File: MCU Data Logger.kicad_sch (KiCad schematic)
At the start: 25 parts, among them U1 24LC1025, U2 24LC1025, U3 DS1337S_, U4 ATmega328P-A, Y1 32.768KHz, Y2 16MHz

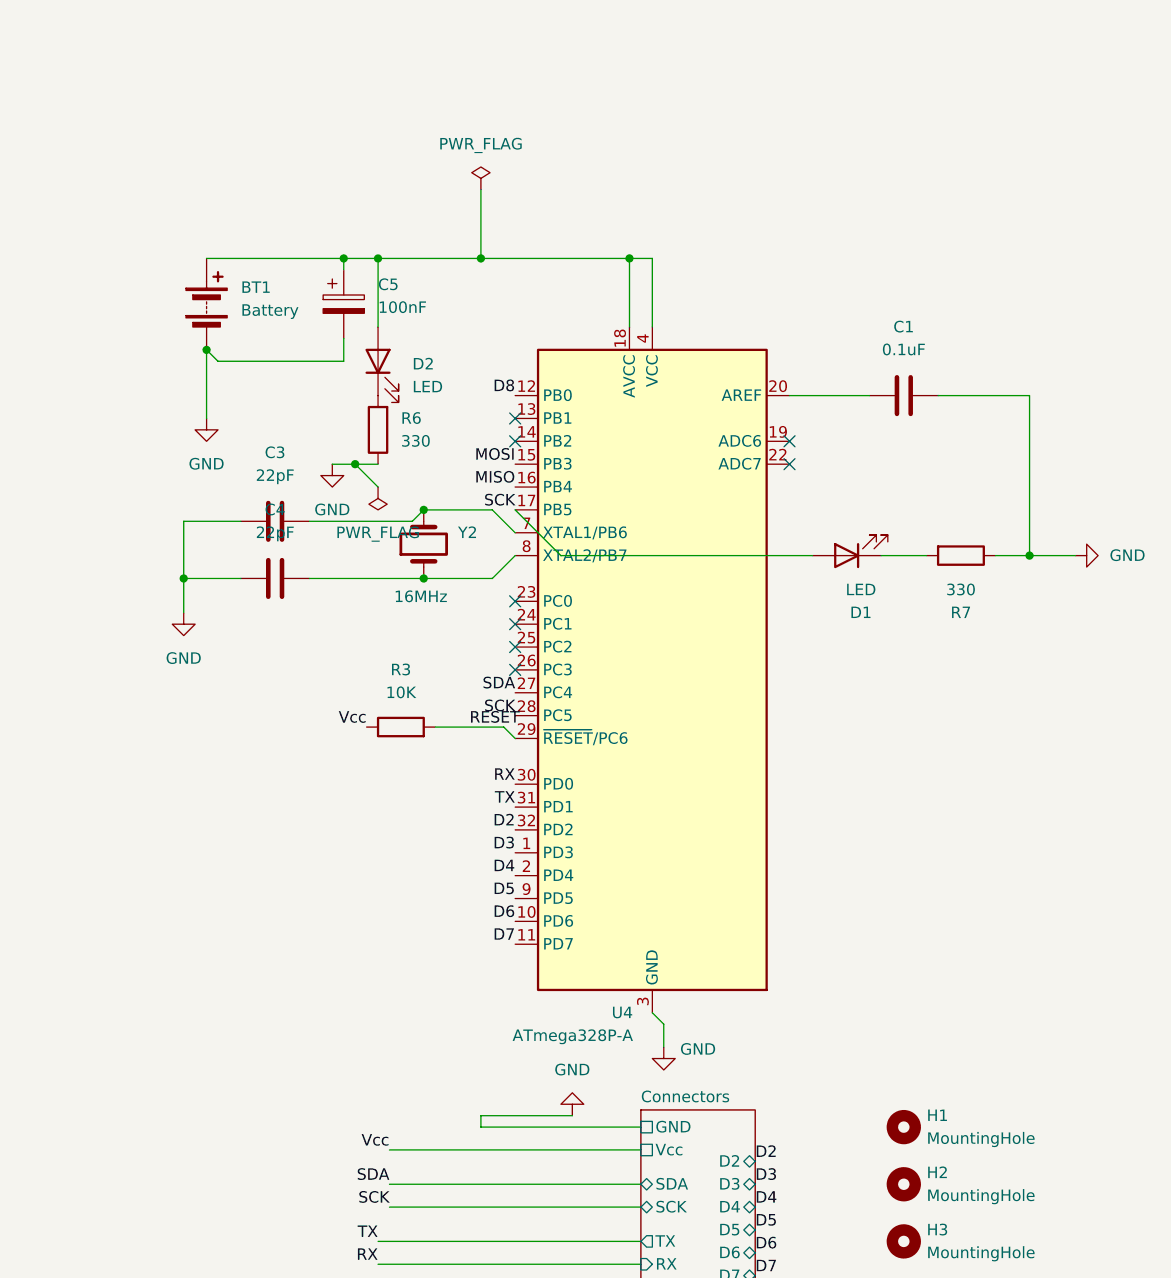
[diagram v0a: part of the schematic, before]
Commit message: complete PCB
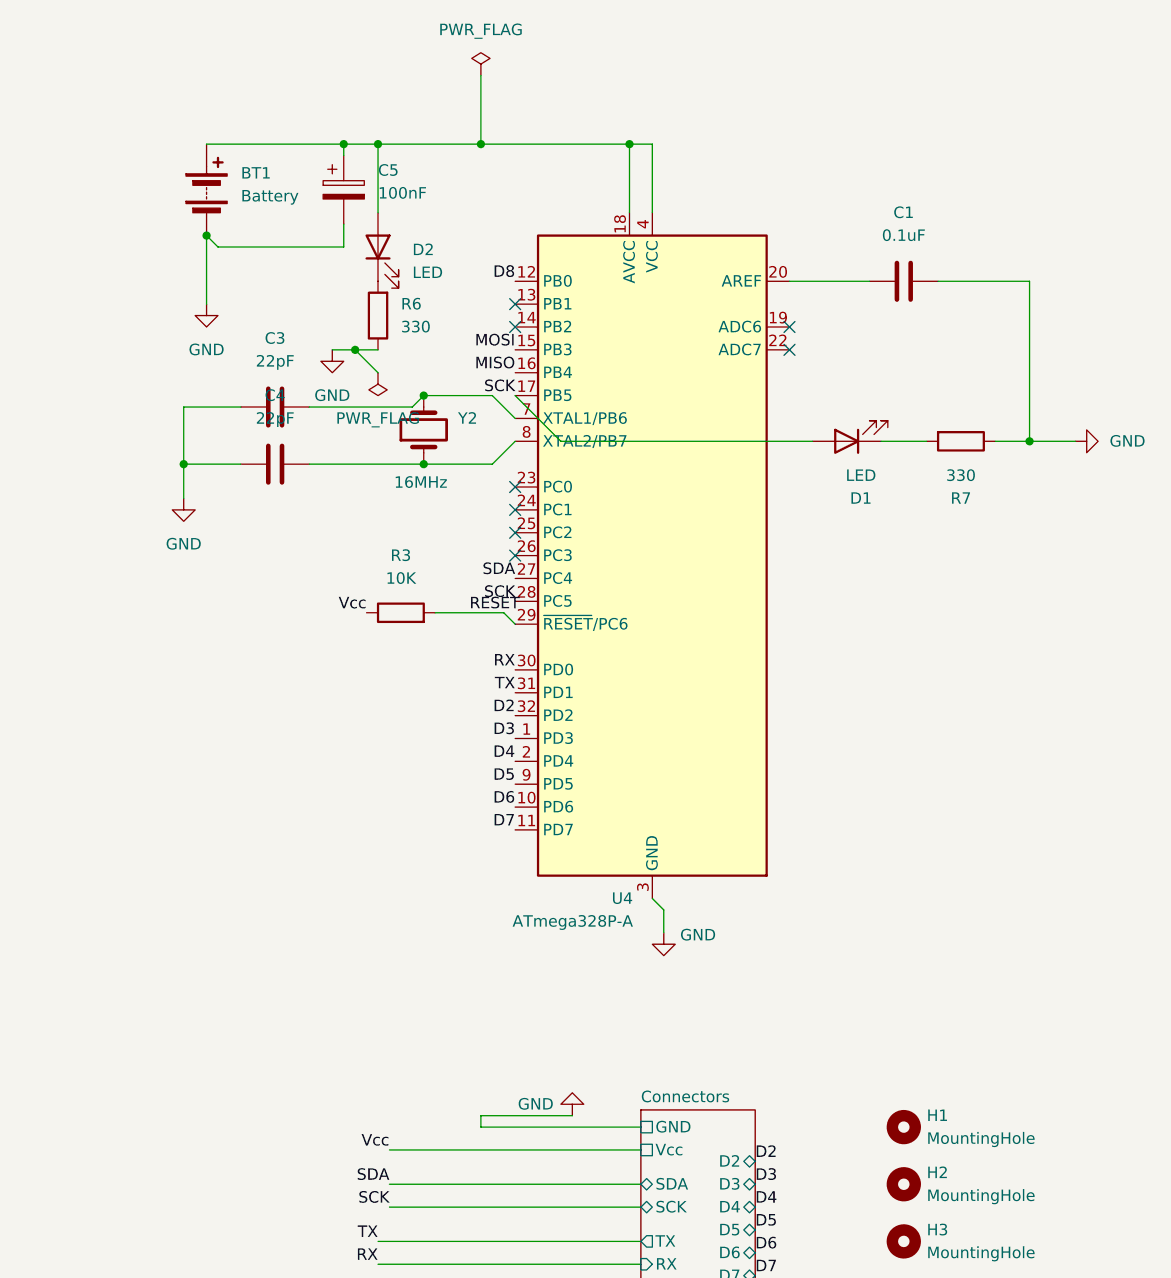
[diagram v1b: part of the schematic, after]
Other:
- moved on the sheet: BT1, C1, C3, C4, C5, D1, D2, R3, R6, R7, U4, Y2
